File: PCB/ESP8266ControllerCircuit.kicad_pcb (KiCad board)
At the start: 2 copper layers, 53.3 x 68.6 mm, 14 parts, among them IC1 SN75176BDR, J1 Transmit, J2 Transmit, U1 JL850B-85003GA1, U2 EL3H7(B)(TA)-G, U3 JL850B-85003GA1, U4 DBT10-7.62-2P-GN

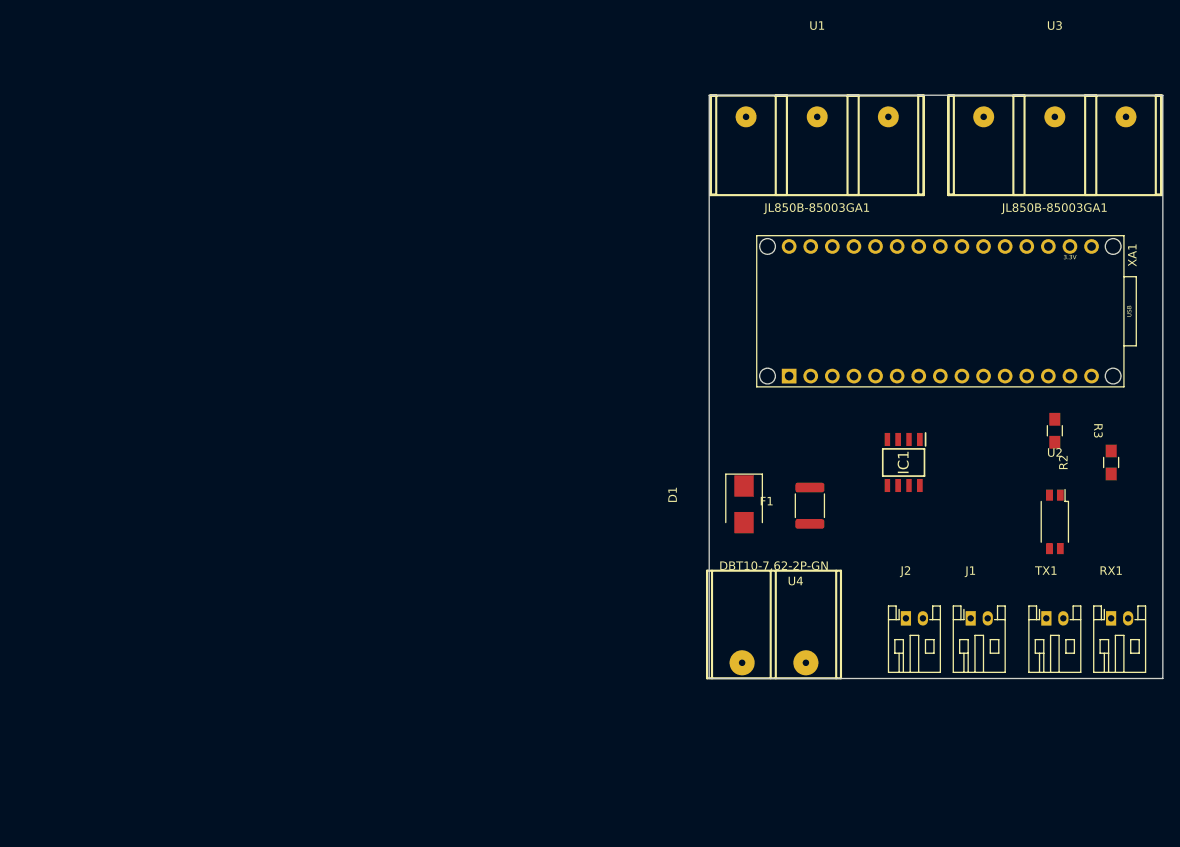
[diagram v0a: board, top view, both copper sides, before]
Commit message: add
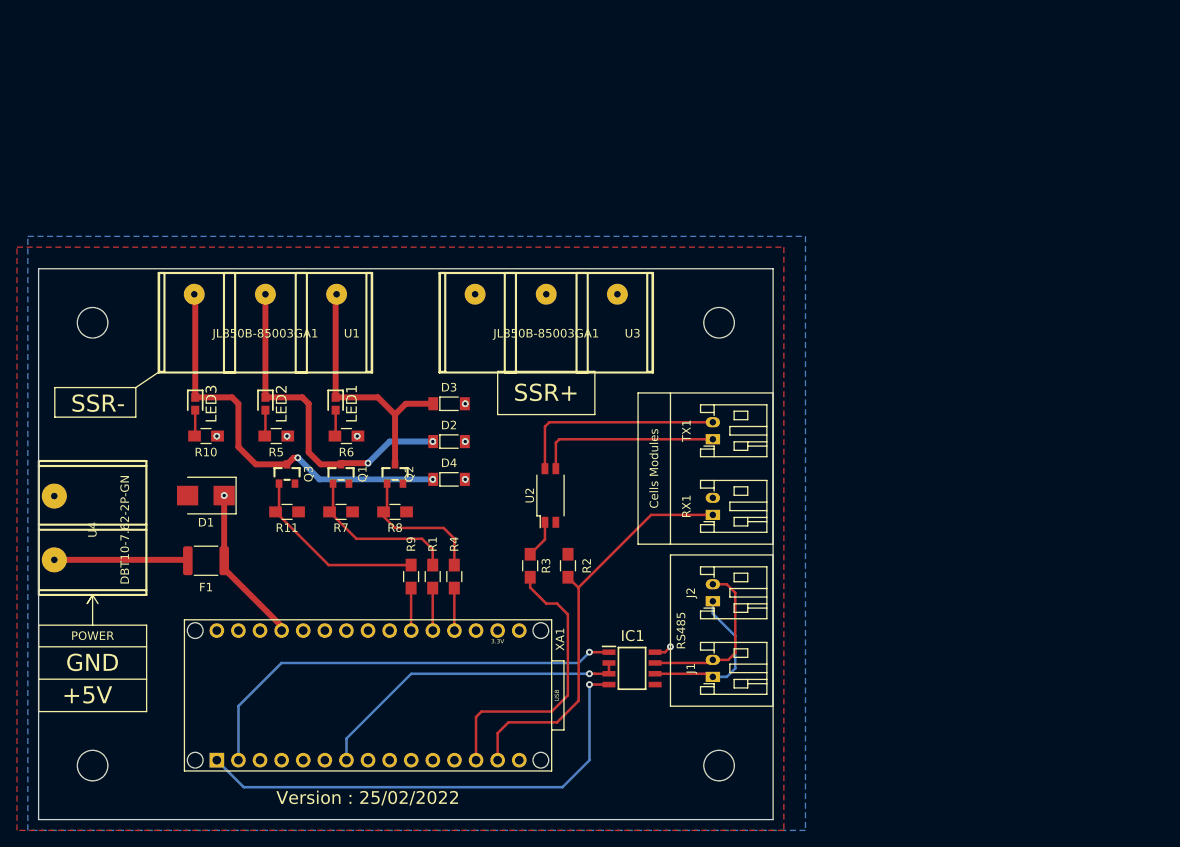
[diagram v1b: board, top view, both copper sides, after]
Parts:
- added D2: LL4148, librarie2:LL4148, F.Cu at (184.2, 71.1)
- added D3: LL4148, librarie2:LL4148, F.Cu at (184.2, 66.7)
- added D4: LL4148, librarie2:LL4148, F.Cu at (184.2, 75.6)
- added LED1: 19-213_Y2C-CQ2R2L_3T_CY_, librarie2:19-213_Y2C-CQ2R2L_3T(CY), F.Cu at (170.8, 66.7)
- added LED2: 19-213_Y2C-CQ2R2L_3T_CY_, librarie2:19-213_Y2C-CQ2R2L_3T(CY), F.Cu at (162.6, 66.7)
- added LED3: 19-213_Y2C-CQ2R2L_3T_CY_, librarie2:19-213_Y2C-CQ2R2L_3T(CY), F.Cu at (154.3, 66.7)
- added Q1: AO3400A, librarie2:AO3400A, F.Cu at (171.4, 74.9)
- added Q2: AO3400A, librarie2:AO3400A, F.Cu at (177.8, 74.9)
- added Q3: AO3400A, librarie2:AO3400A, F.Cu at (165.1, 74.9)
- added R1: 220R, ModuleV440:resistor, F.Cu at (182.2, 87.0)
- added R10: 560, ModuleV440:resistor, F.Cu at (155.6, 70.5)
- added R11: 10K, ModuleV440:resistor, F.Cu at (165.1, 79.4)
- added R4: 220R, ModuleV440:resistor, F.Cu at (184.8, 87.0)
- added R5: 560, ModuleV440:resistor, F.Cu at (163.8, 70.5)
- added R6: 560, ModuleV440:resistor, F.Cu at (172.1, 70.5)
- added R7: 10K, ModuleV440:resistor, F.Cu at (171.4, 79.4)
- added R8: 10K, ModuleV440:resistor, F.Cu at (177.8, 79.4)
- added R9: 220R, ModuleV440:resistor, F.Cu at (179.7, 87.0)
- moved U4 86.1 mm to (137.7, 81.3), turned to 90 degrees
- moved XA1 81.0 mm to (196.2, 101.0)
- moved R3 68.6 mm to (193.7, 85.7), turned to 90 degrees
- moved U1 68.2 mm to (162.6, 53.8)
- moved F1 66.2 mm to (155.6, 85.1)
- moved U3 63.3 mm to (195.6, 53.8)
- moved D1 63.0 mm to (155.6, 77.5), turned to 0 degrees
- moved R2 60.0 mm to (198.1, 85.7)
- moved U2 59.4 mm to (196.2, 77.5), turned to 90 degrees
- moved RX1 45.6 mm to (217.2, 78.7), turned to 90 degrees
- moved TX1 40.9 mm to (217.2, 69.8), turned to 90 degrees
- moved IC1 40.0 mm to (205.7, 97.8), turned to 0 degrees
- moved J1 30.4 mm to (217.2, 97.8), turned to 90 degrees
- moved J2 20.8 mm to (217.2, 88.9), turned to 90 degrees
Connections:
- D1 pad 1: +5V -> R1+
- F1 pad 1: +5V -> R1+
- IC1 pad 8: +5V -> R1+
- RX1 pad 2: +5V -> R1+
- U1 pad 1: GND -> R3-
- U1 pad 2: GND -> R2-
- U1 pad 3: GND -> R1-
- U3 pad 1: Net-(XA1-PadA2) -> R1+
- U3 pad 2: Net-(XA1-PadA1) -> R1+
- U3 pad 3: Net-(XA1-PadA0) -> R1+
- XA1 pad 5V: +5V -> R1+
- XA1 pad A0: Net-(XA1-PadA0) -> Relay1
- XA1 pad A1: Net-(XA1-PadA1) -> Relay2
- XA1 pad A2: Net-(XA1-PadA2) -> Relay3
- XA1 pad D0: unconnected-(XA1-PadD0) -> RS485_RX
- XA1 pad D1: unconnected-(XA1-PadD1) -> RS485_TX
- XA1 pad D2: RS485_EN -> unconnected-(XA1-PadD2)
- XA1 pad D3: RS485_RX -> unconnected-(XA1-PadD3)
- XA1 pad D4: RS485_TX -> RS485_EN
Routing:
- net RS485_TX: track 0.00 -> 57.6 mm, vias 0 -> 1
- net RS485_RX: track 0.00 -> 52.6 mm, vias 0 -> 1
- net Net-(R2-Pad2): track 0.00 -> 48.7 mm
- net R3-: track 0.00 -> 47.8 mm, vias 0 -> 2
- net R2-: track 0.00 -> 39.6 mm, vias 0 -> 2
- net RS485_EN: track 0.00 -> 37.8 mm, vias 0 -> 1
- net Net-(R3-Pad2): track 0.00 -> 33.4 mm
- net R1-: track 0.00 -> 30.9 mm
- net Net-(TX1-Pad2): track 0.00 -> 24.9 mm
- net Net-(Q3-Pad1): track 0.00 -> 22.0 mm
- net Net-(TX1-Pad1): track 0.00 -> 21.7 mm
- net R1+: track 0.00 -> 21.0 mm, vias 0 -> 8
- net Net-(IC1-Pad7): track 0.00 -> 20.0 mm
- net Net-(Q1-Pad1): track 0.00 -> 19.3 mm
- net Net-(IC1-Pad6): track 0.00 -> 19.0 mm
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- added copper zone on F.Cu, net GND
- added copper zone on B.Cu, net R1+
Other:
- board size 53.3 x 68.6 mm -> 86.4 x 64.8 mm
- rule pad_to_mask_clearance: 0.051 -> 0
- board text added: "+5V"
- board text added: "Cells Modules"
- board text added: "GND"
- board text added: "POWER"
- board text added: "RS485"
- board text added: "SSR+"
- board text added: "SSR-"
- board text added: "Version : 25/02/2022"
